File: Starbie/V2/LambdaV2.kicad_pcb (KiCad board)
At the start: 2 copper layers, 136.5 x 108 mm, 21 parts, among them J1 Conn_01x04_Pin, J2 Conn_01x08_Pin, J3 Conn_01x05_Pin, P1 USB_C_Plug_USB2.0, SW1 SW_Push, SW2 SW_Push, SW3 SW_Push, SW4 SW_Omron_B3FS, SW5 SW_Omron_B3FS, SW7 RotaryEncoder_Switch, U1 ESP32-C6-DevKitC-1, U2 AM2302

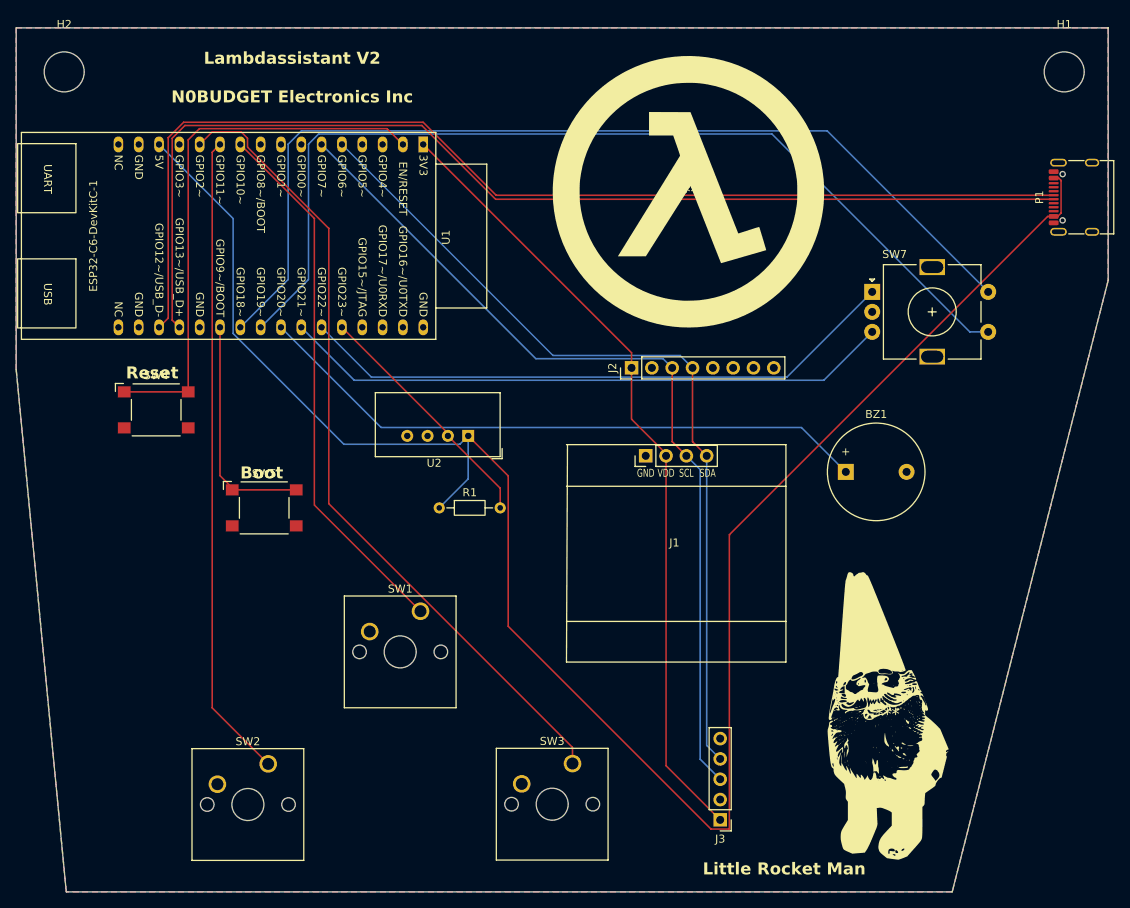
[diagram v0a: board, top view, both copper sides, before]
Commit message: updated buttons and stuff
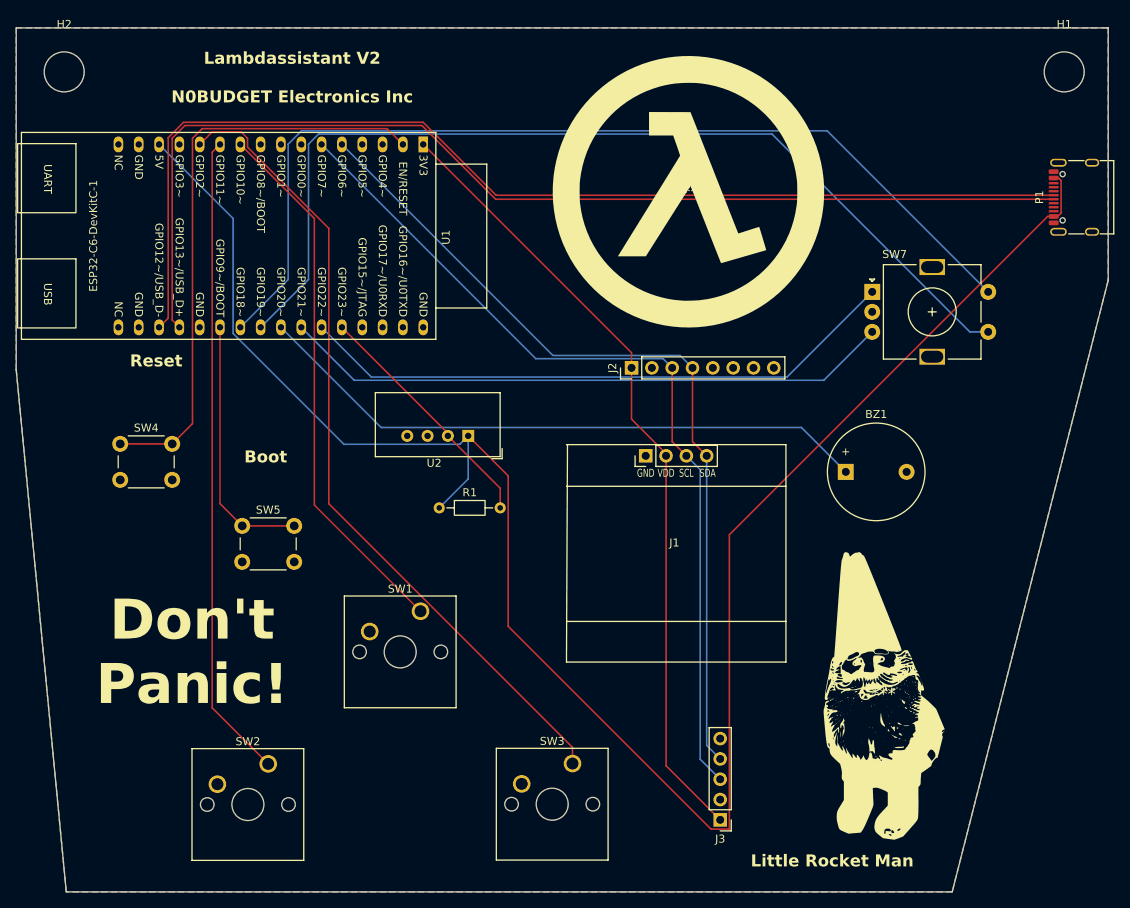
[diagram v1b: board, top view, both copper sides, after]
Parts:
- SW4, SW5: value SW_Omron_B3FS -> SW_Push; footprint Button_Switch_SMD:SW_SPST_Omron_B3FS-100xP -> Button_Switch_THT:SW_PUSH_6mm_H5mm
- moved SW4 6.19 mm to (82.0, 92.0)
- moved SW5 3.55 mm to (97.2, 102.2)
- moved G*** 2.55 mm to (176.6, 123.3)
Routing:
- net /RST: track 67.7 -> 73.4 mm
- net /BOOT: track 29.0 -> 32.5 mm
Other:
- board text added: "Don't Panic!"
